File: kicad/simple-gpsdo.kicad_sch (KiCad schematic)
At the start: 33 parts, among them J1 ISP, J2 Barrel_Jack, P1 USB_C_Plug_USB2.0, Q1 AO3401A, SW1 RESET, U1 ATmega328P-A, U2 FT231XQ, U3 REF3040, U4 XRP6272ITC5TR-F, U6 TPS5430DDA, Y1 16 MHz

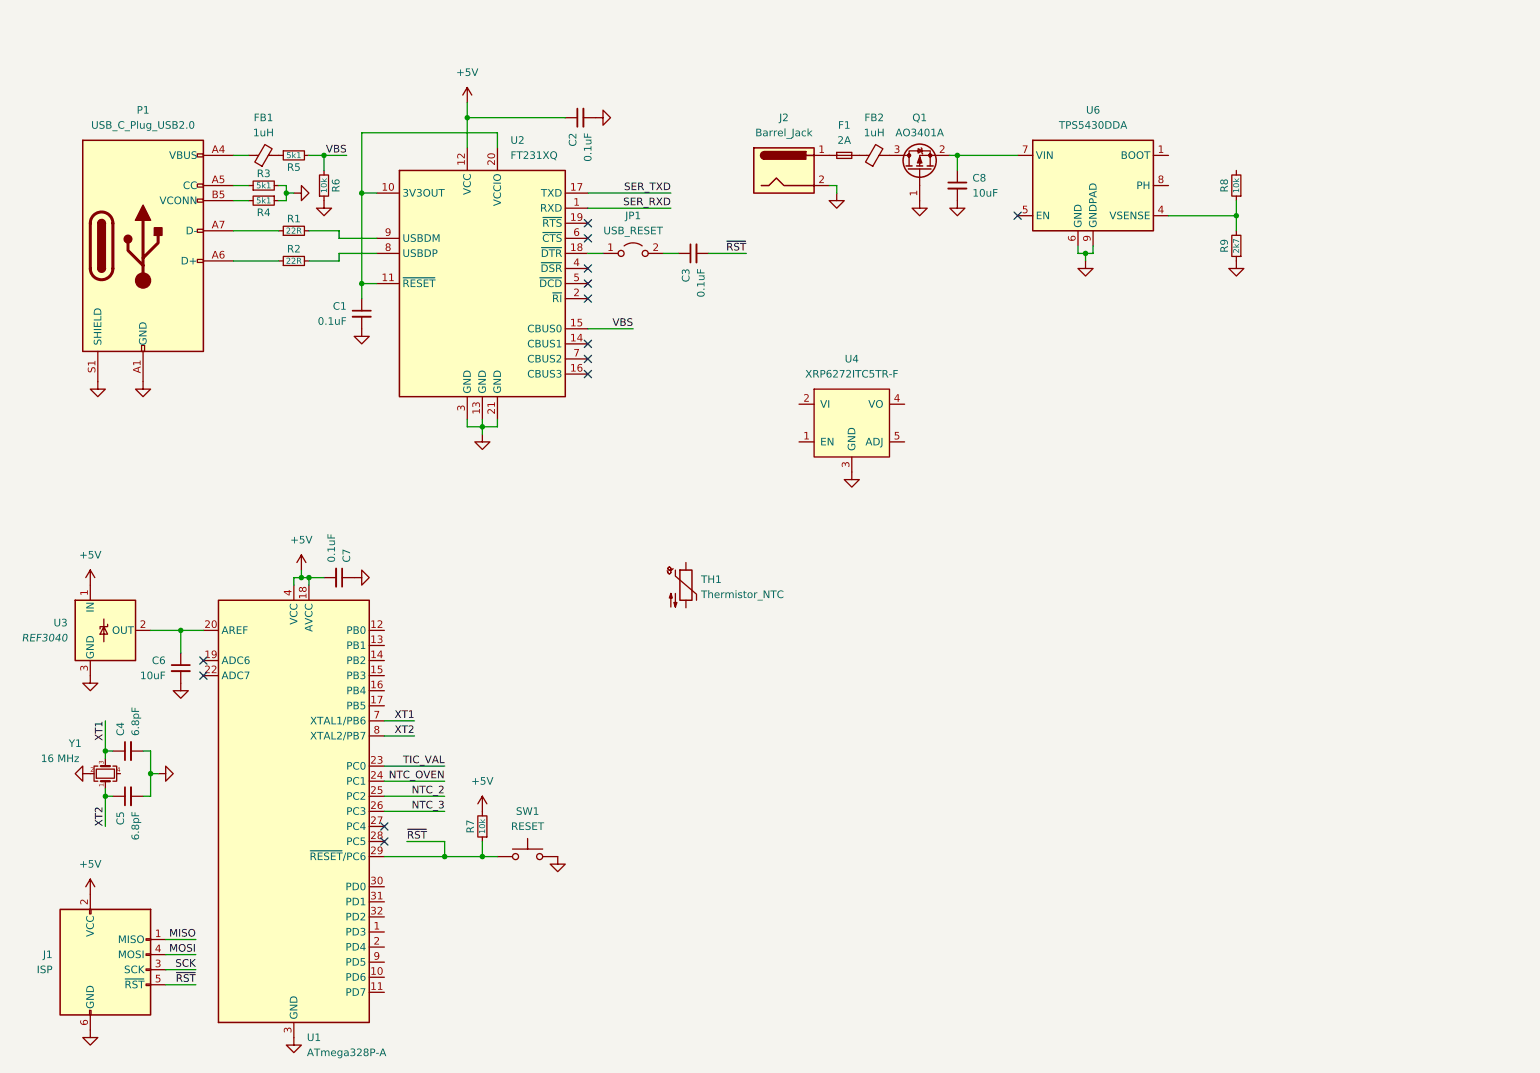
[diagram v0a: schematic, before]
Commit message: more work on schematic
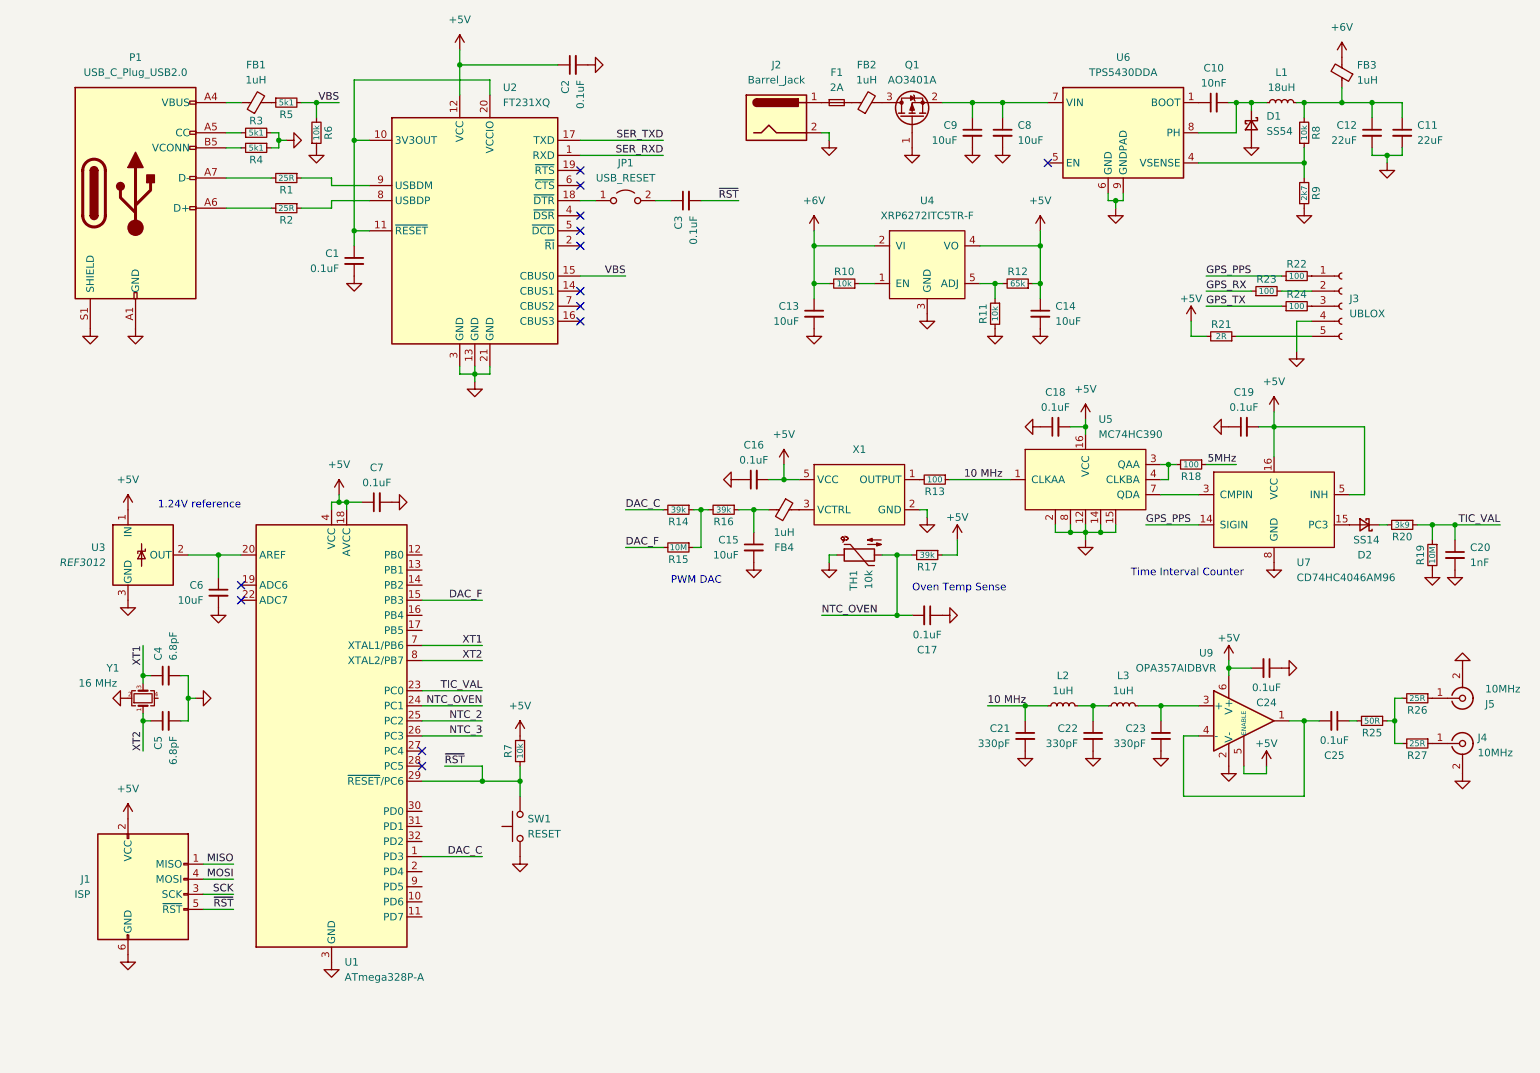
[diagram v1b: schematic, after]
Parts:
- removed U3: REF3040, Package_TO_SOT_SMD:SOT-23, symbol Reference_Voltage:REF3040
- added C10: 10nF, symbol Device:C_Small
- added C11, C12: 22uF, symbol Device:C_Small
- added C13, C14, C15, C9: 10uF, symbol Device:C_Small
- added C16, C17, C18, C19, C24, C25: 0.1uF, symbol Device:C_Small
- added C20: 1nF, symbol Device:C_Small
- added C21, C22, C23: 330pF, symbol Device:C_Small
- added D1: SS54, Diode_SMD:D_SMA, symbol Device:D_Schottky_Small
- added D2: SS14, Diode_SMD:D_SMA, symbol Device:D_Schottky_Small
- added FB3, FB4: 1uH, symbol Device:FerriteBead_Small
- added J3: UBLOX, symbol Connector:Conn_01x05_Socket
- added J4, J5: 10MHz, symbol Connector:Conn_Coaxial
- added L1: 18uH, symbol Device:L_Small
- added L2, L3: 1uH, symbol Device:L_Small
- added R10, R11: 10k, symbol Device:R_Small
- added R12: 65k, symbol Device:R_Small
- added R13, R18, R22, R23, R24: 100, symbol Device:R_Small
- added R14, R16, R17: 39k, symbol Device:R_Small
- added R15, R19: 10M, symbol Device:R_Small
- added R20: 3k9, symbol Device:R_Small
- added R21: 2R, symbol Device:R_Small
- added R25: 50R, symbol Device:R_Small
- added R26, R27: 25R, symbol Device:R_Small
- added U3: REF3012, Package_TO_SOT_SMD:SOT-23, symbol Reference_Voltage:REF3012
- added U5: MC74HC390, symbol 74HC:MC74HC390
- added U7: CD74HC4046AM96, symbol 74HC:CD74HC4046AM96
- added U9: OPA357AIDBVR, Package_TO_SOT_SMD:SOT-23-6, symbol Amplifier_Operational:OPA355NA
- added X1: ~, symbol ocxo:OCXO-5PIN
- R1, R2: value 22R -> 25R
- TH1: value Thermistor_NTC -> 10k
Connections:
- net +5V: now also C7.1, U4.4 (VO), C14.1, C16.2, C18.2, C19.2, C24.2, R12.1, R17.1, R21.2, U3.1 (IN), U5.16 (VCC), U7.16 (VCC), U7.5 (INH), U9.5 (ENABLE), U9.6 (V+), X1.5 (VCC); no longer C7.2
- net GND: now also C7.2, SW1.1, TH1.1, C11.2, C12.2, C13.2, C14.2, C15.2, C16.1, C17.1, C18.1, C19.1, C20.2, C21.2, C22.2, C23.2, C24.1, C9.2, D1.2 (A), J3.4 (Pin_4), J4.2 (Ext), J5.2 (Ext), R11.2, R19.2, U3.3 (GND), U5.12, U5.14, U5.15, U5.2, U5.8, U7.8 (GND), U9.2 (V-), X1.2 (GND); no longer C7.1, SW1.2
- net NTC_OVEN: now also TH1.2, C17.2, R17.2
- net TIC_VAL: now also C20.1, R19.1, R20.1
- net ~{RST}: now also SW1.2; no longer SW1.1
- net at C8.1, Q1.2 (S), U6.7 (VIN): now also C9.1
- net DAC_C: now reaches U1.1 (PD3)
- net DAC_C: now also R14.2
- net DAC_F: now reaches U1.15 (PB3)
- net DAC_F: now also R15.2
- net at C6.1, U1.20 (AREF): now also U3.2 (OUT)
- net at U6.1 (BOOT): now also C10.1
- net at U6.8 (PH): now also C10.2, D1.1 (K), L1.1
- net at R8.2: now also C11.1, C12.1, FB3.1, L1.2
- net at U2.8 (USBDP): now also R2.1; no longer R2.2
- net at U2.9 (USBDM): now also R1.1; no longer R1.2
- net at P1.A6 (D+): now also R2.2; no longer R2.1
- net at P1.A7 (D-): now also R1.2; no longer R1.1
- net at U4.1 (EN): now also R10.1
- net +6V: now reaches U4.2 (VI)
- net +6V: now also C13.1, FB3.2, R10.2
- net at U4.5 (ADJ): now also R11.1, R12.2
- new net: R18.2, U5.3 (QAA), U5.4 (CLKBA)
- new net: J5.1 (In), R26.1
- new net: R25.1, R26.2, R27.2
- new net: J3.1 (Pin_1), R22.2
- new net: C15.1, FB4.2, R16.1
- new net: R14.1, R15.1, R16.2
- new net: D2.1 (K), R20.2
- new net: J4.1 (In), R27.1
- new net: C25.1, R25.2
- new net: R13.2, X1.1 (OUTPUT)
- new net: FB4.1, X1.3 (VCTRL)
- new net: U5.7 (QDA), U7.3 (CMPIN)
- new net: D2.2 (A), U7.15 (PC3)
- new net: C25.2, U9.1, U9.4 (-)
- new net: C23.1, L3.2, U9.3 (+)
- new net: J3.2 (Pin_2), R23.2
- new net: J3.3 (Pin_3), R24.2
- new net: J3.5 (Pin_5), R21.1
- new net: C22.1, L2.2, L3.1
- new net 10 MHz: C21.1, L2.1, R13.1, U5.1 (CLKAA)
- new net 5MHz: R18.1
- new net GPS_PPS: R22.1, U7.14 (SIGIN)
- new net GPS_RX: R23.1
- new net GPS_TX: R24.1
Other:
- note added: "1.24V reference"
- note added: "Oven Temp Sense"
- note added: "PWM DAC"
- note added: "Time Interval Counter"
- moved on the sheet: C1, C2, C3, C4, C5, C6, C8, F1, FB1, FB2, J1, J2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
